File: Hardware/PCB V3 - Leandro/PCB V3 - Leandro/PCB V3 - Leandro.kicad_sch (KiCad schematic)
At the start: 15 parts, among them J10 MOTOR_DER, J3 Sensor TATAMI FD, J4 SWITCH, J5 Sensor TATAMI FI, J6 STEP_DOWN, J7 IR_FD, J8 IR_FI, J9 MOTOR_IZQ, SW1 START, SW2 ESTRATEGIA, U1 ESP32_DevKit_V1_CH9102X

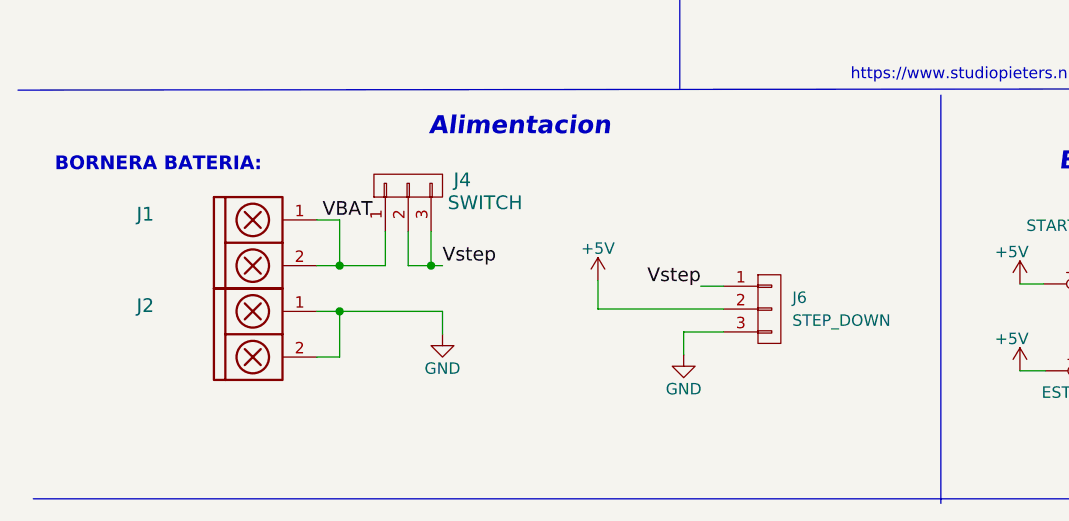
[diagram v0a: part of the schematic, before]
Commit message: falta la correccion de Bustos y diseñar el svg
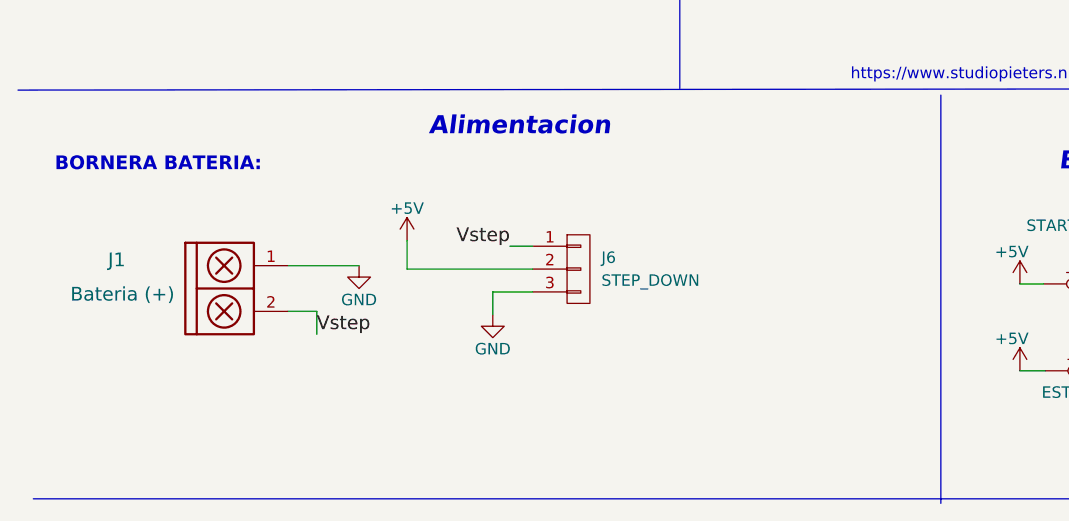
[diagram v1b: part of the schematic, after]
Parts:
- removed J2: (no value), EESTN5:BORNERA2_AZUL, symbol EESTN5:TB_1X2
- removed J4: SWITCH, EESTN5:SW_SPDT_TH_Vertical, symbol EESTN5:Conn_01X03
- J1: value (none) -> Bateria (+)
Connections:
- net GND: now also J1.1
- net Vstep: now also J1.2
- removed net VBAT: J1.1, J1.2
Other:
- moved on the sheet: J1, J6
